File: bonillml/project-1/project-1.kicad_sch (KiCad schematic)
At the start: 7 parts, among them J1 Conn_01x04

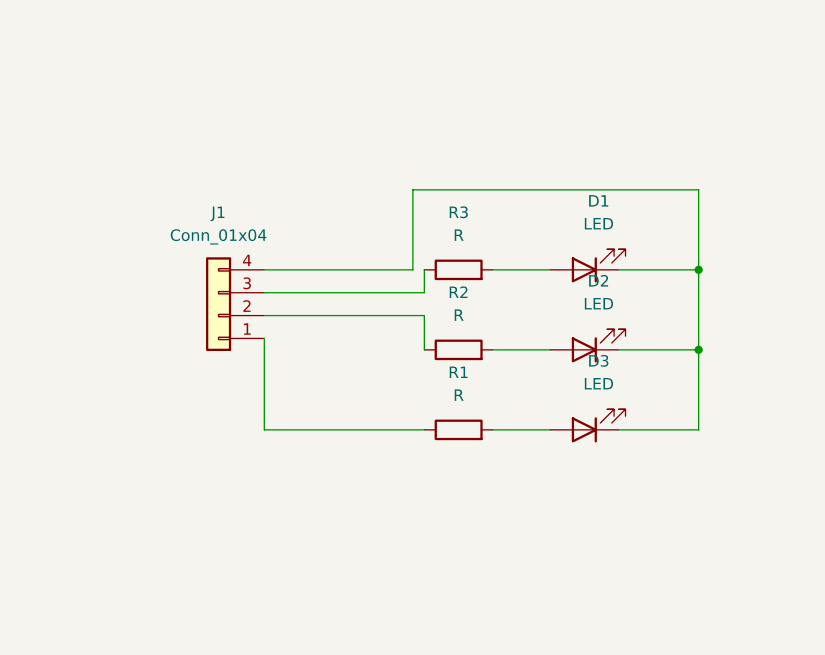
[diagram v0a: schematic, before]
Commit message: Boinkers (CAN)
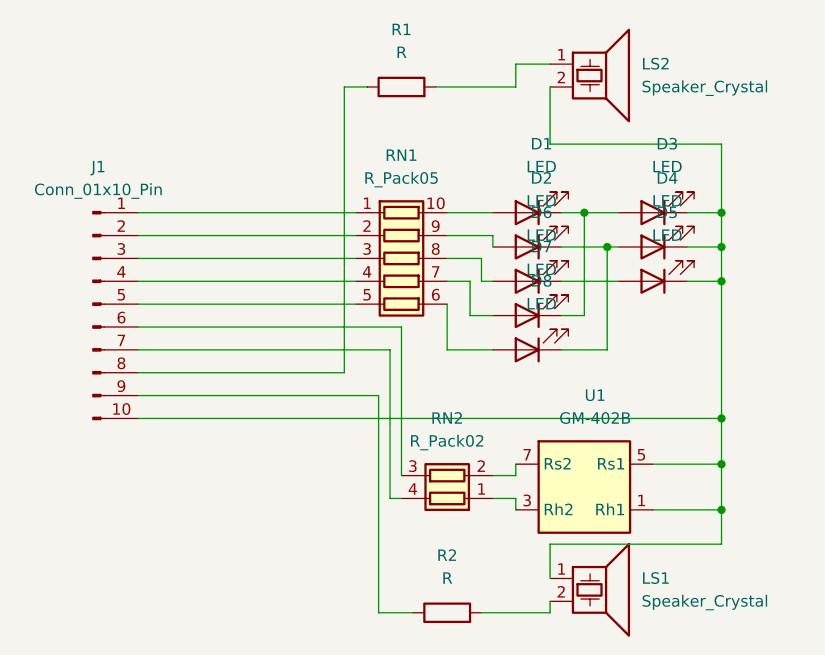
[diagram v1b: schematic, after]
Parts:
- removed J1: Conn_01x04, Connector_PinHeader_2.00mm:PinHeader_1x04_P2.00mm_Horizontal, symbol Connector_Generic:Conn_01x04
- removed R3: R, Resistor_THT:R_Axial_DIN0411_L9.9mm_D3.6mm_P15.24mm_Horizontal, symbol Device:R
- added D4, D5, D6, D7, D8: LED, LED_THT:LED_D5.0mm_Horizontal_O6.35mm_Z9.0mm, symbol Device:LED
- added J1: Conn_01x10_Pin, Connector:Connector_SFP_and_Cage, symbol Connector:Conn_01x10_Pin
- added LS1, LS2: Speaker_Crystal, Crystal:Crystal_HC18-U_Vertical, symbol Device:Speaker_Crystal
- added RN1: R_Pack05, Resistor_THT:R_Array_SIP14, symbol Device:R_Pack05
- added RN2: R_Pack02, Resistor_THT:R_Array_SIP14, symbol Device:R_Pack02
- added U1: GM-402B, Sensor:Winson_GM-402B_5x5mm_P1.27mm, symbol Sensor_Gas:GM-402B
- D1, D2, D3: footprint LED_THT:LED_D3.0mm -> LED_THT:LED_D5.0mm_Horizontal_O6.35mm_Z9.0mm
- R1, R2: footprint Resistor_THT:R_Axial_DIN0411_L9.9mm_D3.6mm_P15.24mm_Horizontal -> Resistor_THT:R_Axial_DIN0204_L3.6mm_D1.6mm_P7.62mm_Horizontal
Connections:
- net at R2.1: now also J1.9 (Pin_9)
- net at R2.2: now also LS1.2; no longer D2.2 (A)
- net at R1.1: now also J1.8 (Pin_8)
- net at D1.2 (A): now also RN1.10 (R1.2)
- net at D3.2 (A): now also D1.1 (K), D7.1 (K); no longer R1.2
- new net: D5.2 (A), D6.1 (K)
- new net: D6.2 (A), RN1.8 (R3.2)
- new net: RN2.1 (R1.1), U1.3 (Rh2)
- new net: RN2.2 (R2.1), U1.7 (Rs2)
- new net: J1.6 (Pin_6), RN2.3 (R2.2)
- new net: J1.7 (Pin_7), RN2.4 (R1.2)
- new net: D2.1 (K), D4.2 (A), D8.1 (K)
- new net: D8.2 (A), RN1.6 (R5.2)
- new net: D3.1 (K), D4.1 (K), D5.1 (K), J1.10 (Pin_10), LS1.1, LS2.2, U1.1 (Rh1), U1.5 (Rs1)
- new net: D7.2 (A), RN1.7 (R4.2)
- new net: J1.1 (Pin_1), RN1.1 (R1.1)
- new net: J1.2 (Pin_2), RN1.2 (R2.1)
- new net: J1.3 (Pin_3), RN1.3 (R3.1)
- new net: J1.4 (Pin_4), RN1.4 (R4.1)
- new net: J1.5 (Pin_5), RN1.5 (R5.1)
- new net: D2.2 (A), RN1.9 (R2.2)
- new net: LS2.1, R1.2
